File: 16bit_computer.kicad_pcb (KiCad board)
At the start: 2 copper layers, 219.1 x 157.5 mm, 97 parts, among them J1 Conn_01x03, J10 Conn_01x08, J11 Conn_01x08, J12 Conn_01x08, J2 Conn_01x16_Male, J3 Conn_01x08, J4 Conn_01x08, J5 Conn_01x08, J6 Conn_01x08, J7 Conn_01x16, J8 Conn_01x16, J9 Conn_01x08, U1 40374, U10 40374, U11 40374, U12 40245, U13 40245, U14 40374, U15 40374, U16 40245, U17 40245, U2 40374, U3 40245, U4 40245, U5 7408, U6 40374, U7 40374, U8 40245, U9 40245

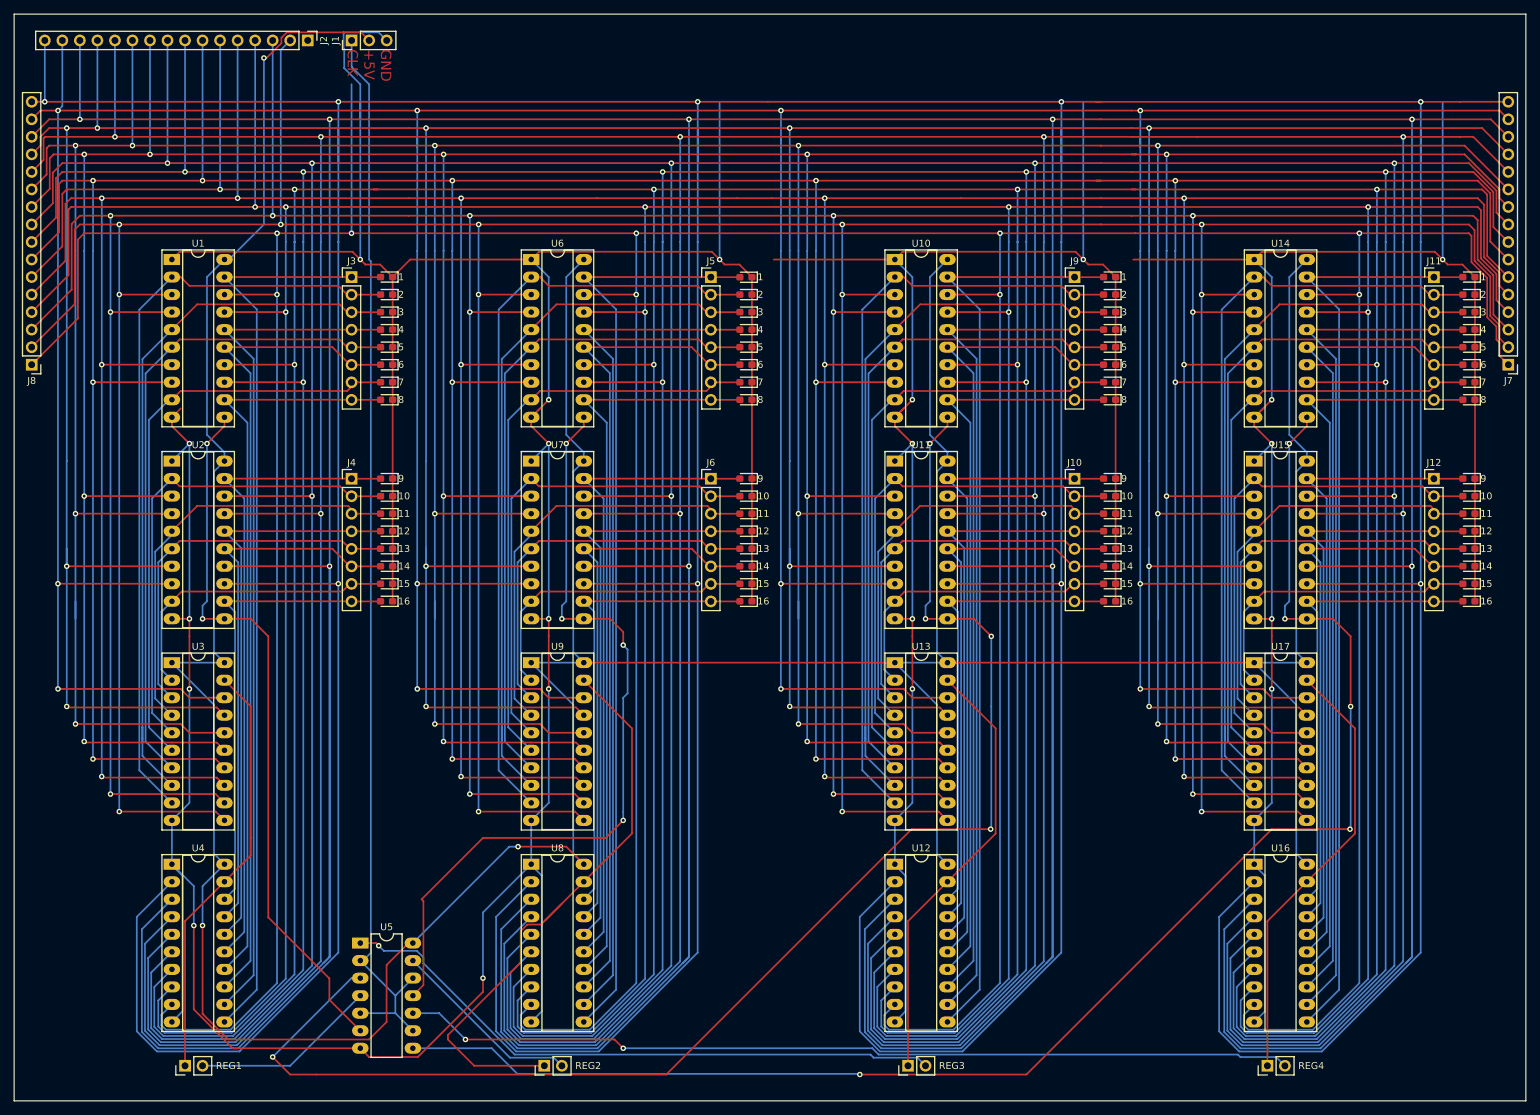
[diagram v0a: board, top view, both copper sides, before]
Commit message: final v0.3
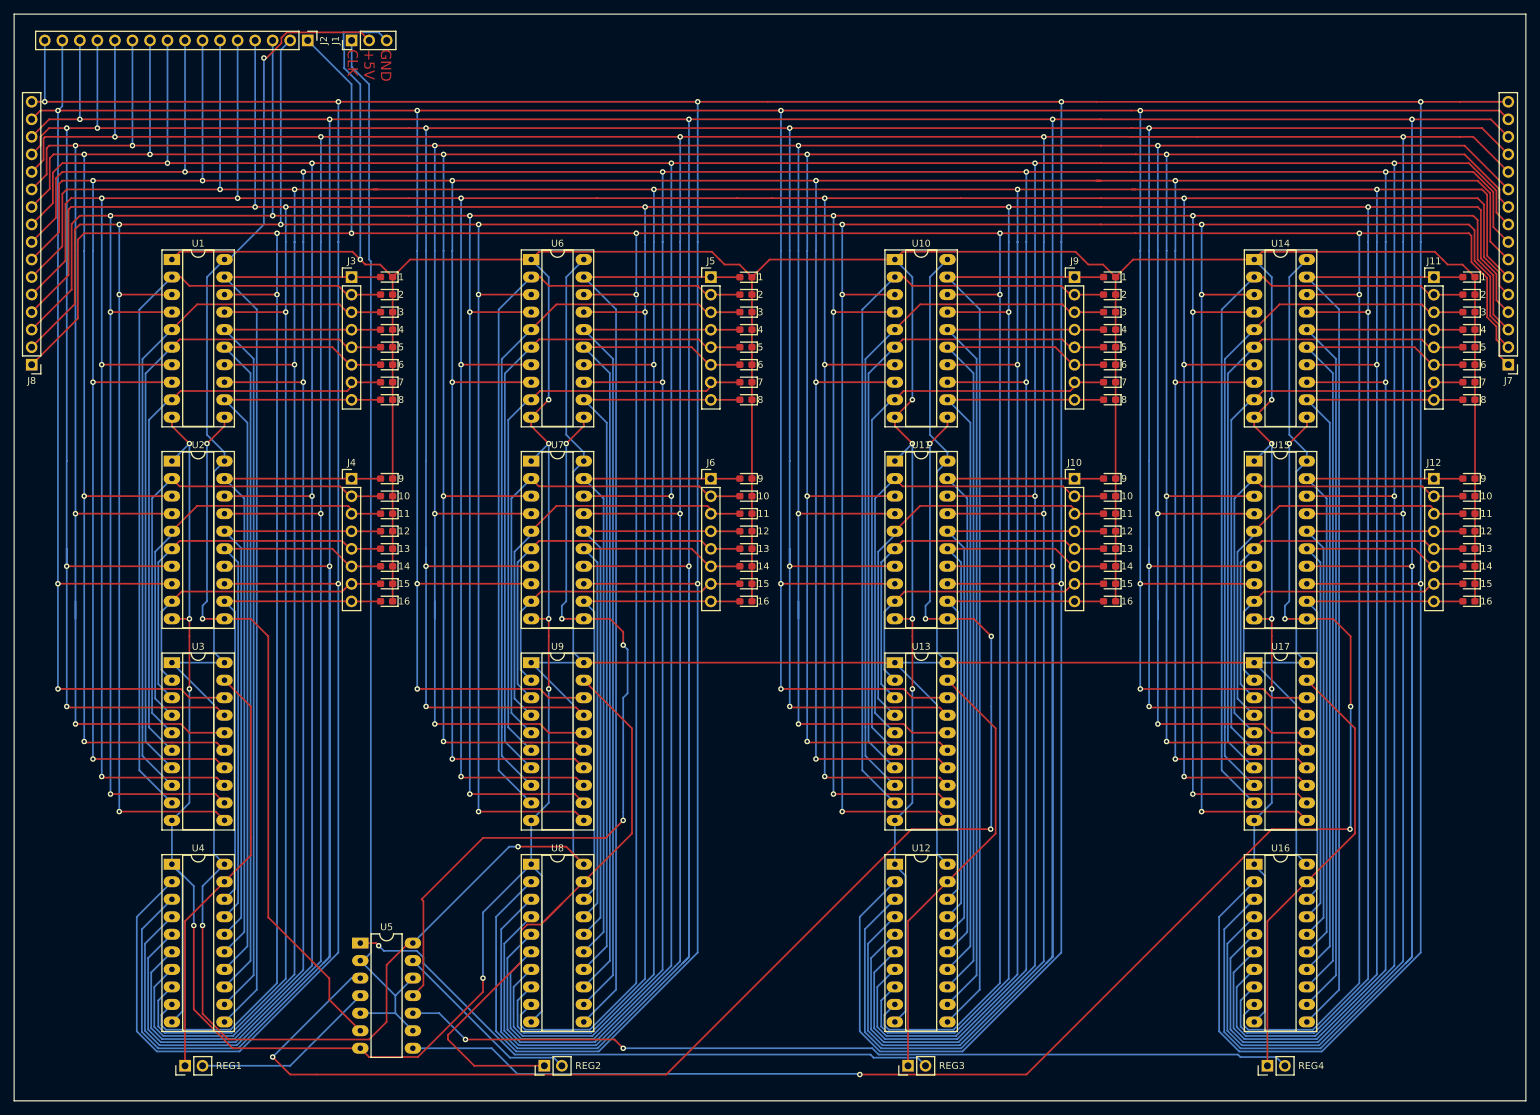
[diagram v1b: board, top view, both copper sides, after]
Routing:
- net GND: track 1055.4 -> 984.5 mm, vias 21 -> 18
- net /BUS16: track 1043.8 -> 1022.8 mm
- net /BUS1: track 825.0 -> 834.0 mm
- net /BUS15: track 731.5 -> 725.5 mm
- net /Register4/data3: track 103.8 -> 101.6 mm
- net /Register3/data3: track 103.8 -> 101.6 mm
- net /Register2/data3: track 103.8 -> 101.6 mm
- net /Register1/data3: track 103.8 -> 101.6 mm
- net +5V: track 645.5 -> 643.6 mm
- net /BUS10: track 715.5 -> 714.8 mm
- net Net-(REG4-Pad2): track 130.1 -> 129.5 mm
